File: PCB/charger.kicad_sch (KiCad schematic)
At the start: 17 parts, among them U2 BQ24072RGT

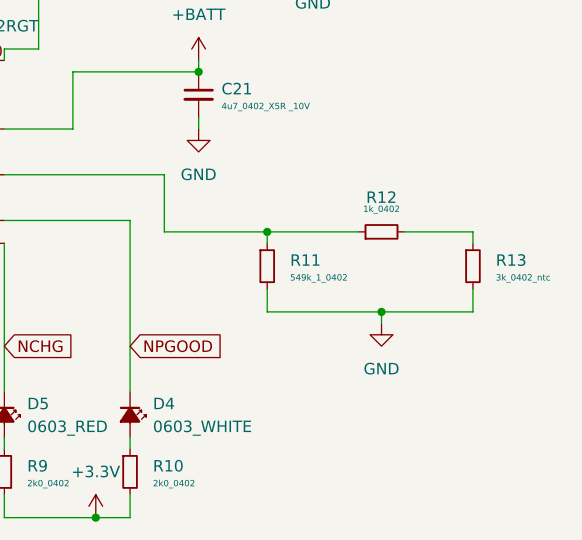
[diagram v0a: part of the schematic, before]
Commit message: Wichtige Änderungen für die Fertigung
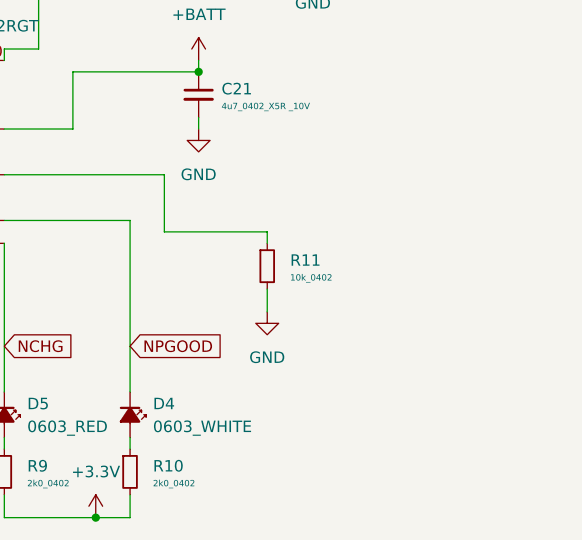
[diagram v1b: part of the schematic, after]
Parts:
- removed R11: 549k_1_0402, Resistor_SMD:R_0402_1005Metric, symbol resistor_smd_extended:549k_1_0402
- removed R12: 1k_0402, Resistor_SMD:R_0402_1005Metric, symbol resistor_smd_standard:1k_0402
- removed R13: 3k_0402_ntc, Resistor_SMD:R_0402_1005Metric, symbol 2_ntc:3k_0402_ntc
- added R11: 10k_0402, Resistor_SMD:R_0402_1005Metric, symbol resistor_smd_standard:10k_0402
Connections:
- net GND: now also R11.2
- net at U2.1 (TS): now also R11.1
